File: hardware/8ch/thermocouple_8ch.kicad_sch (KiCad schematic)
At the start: 167 parts, among them J1 24V_INPUT, J2 LCD_16x2_HEADER, J3 RELAY_COM_NO_NC, J4 RS485_A_B_GND_SHIELD, J5 AVR_ISP, J6 MCU_EXPANSION, K1 G5LE-1 DC24, Q1 2N7000, SW1 NEXT, SW2 UP, SW3 DOWN, SW4 SET, SW5 ACK, U1 ATmega32A-PU, U10 ISO7760FDWR, U11 ISO7761FDWR, U12 IA0505S, U13 LP2985-3.3, U14 TSR 1-2450, U15 ADM2587EBRWZ, U2 MAX31856MUD+, U3 MAX31856MUD+, U4 MAX31856MUD+, U5 MAX31856MUD+, U6 MAX31856MUD+, U7 MAX31856MUD+, U8 MAX31856MUD+, U9 MAX31856MUD+

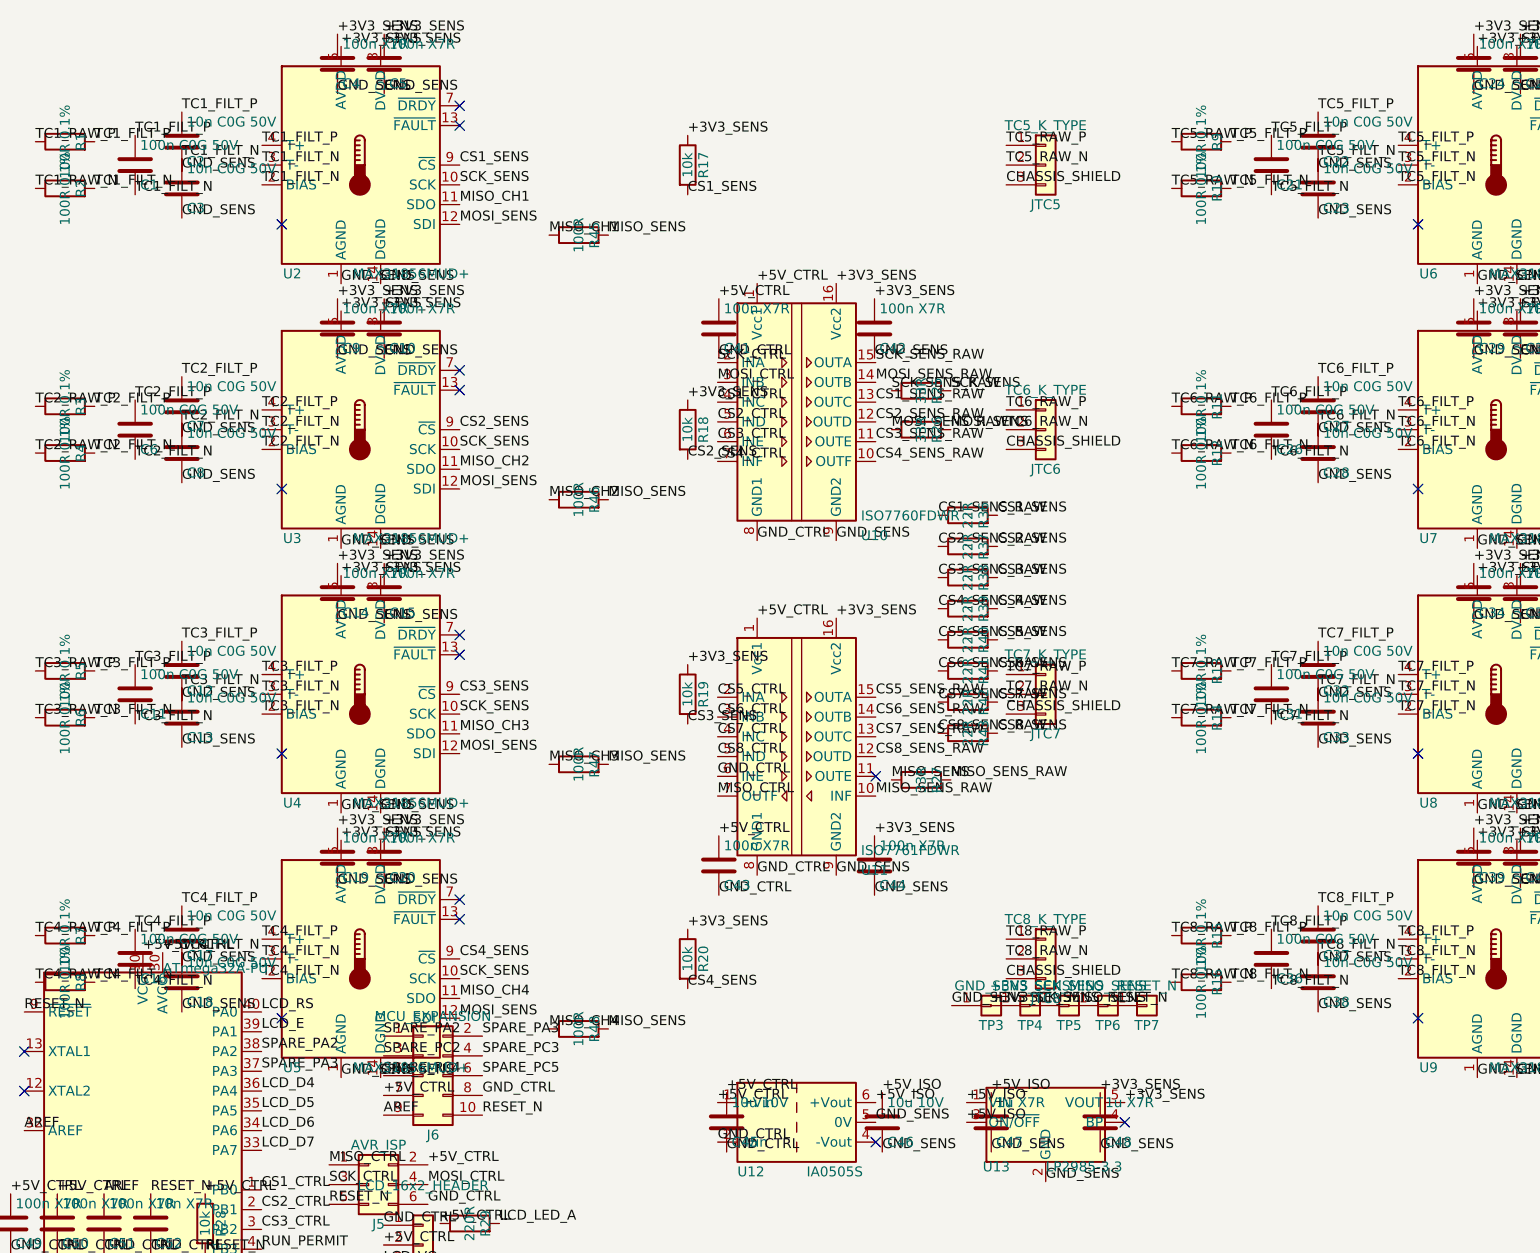
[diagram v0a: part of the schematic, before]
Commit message: tools config
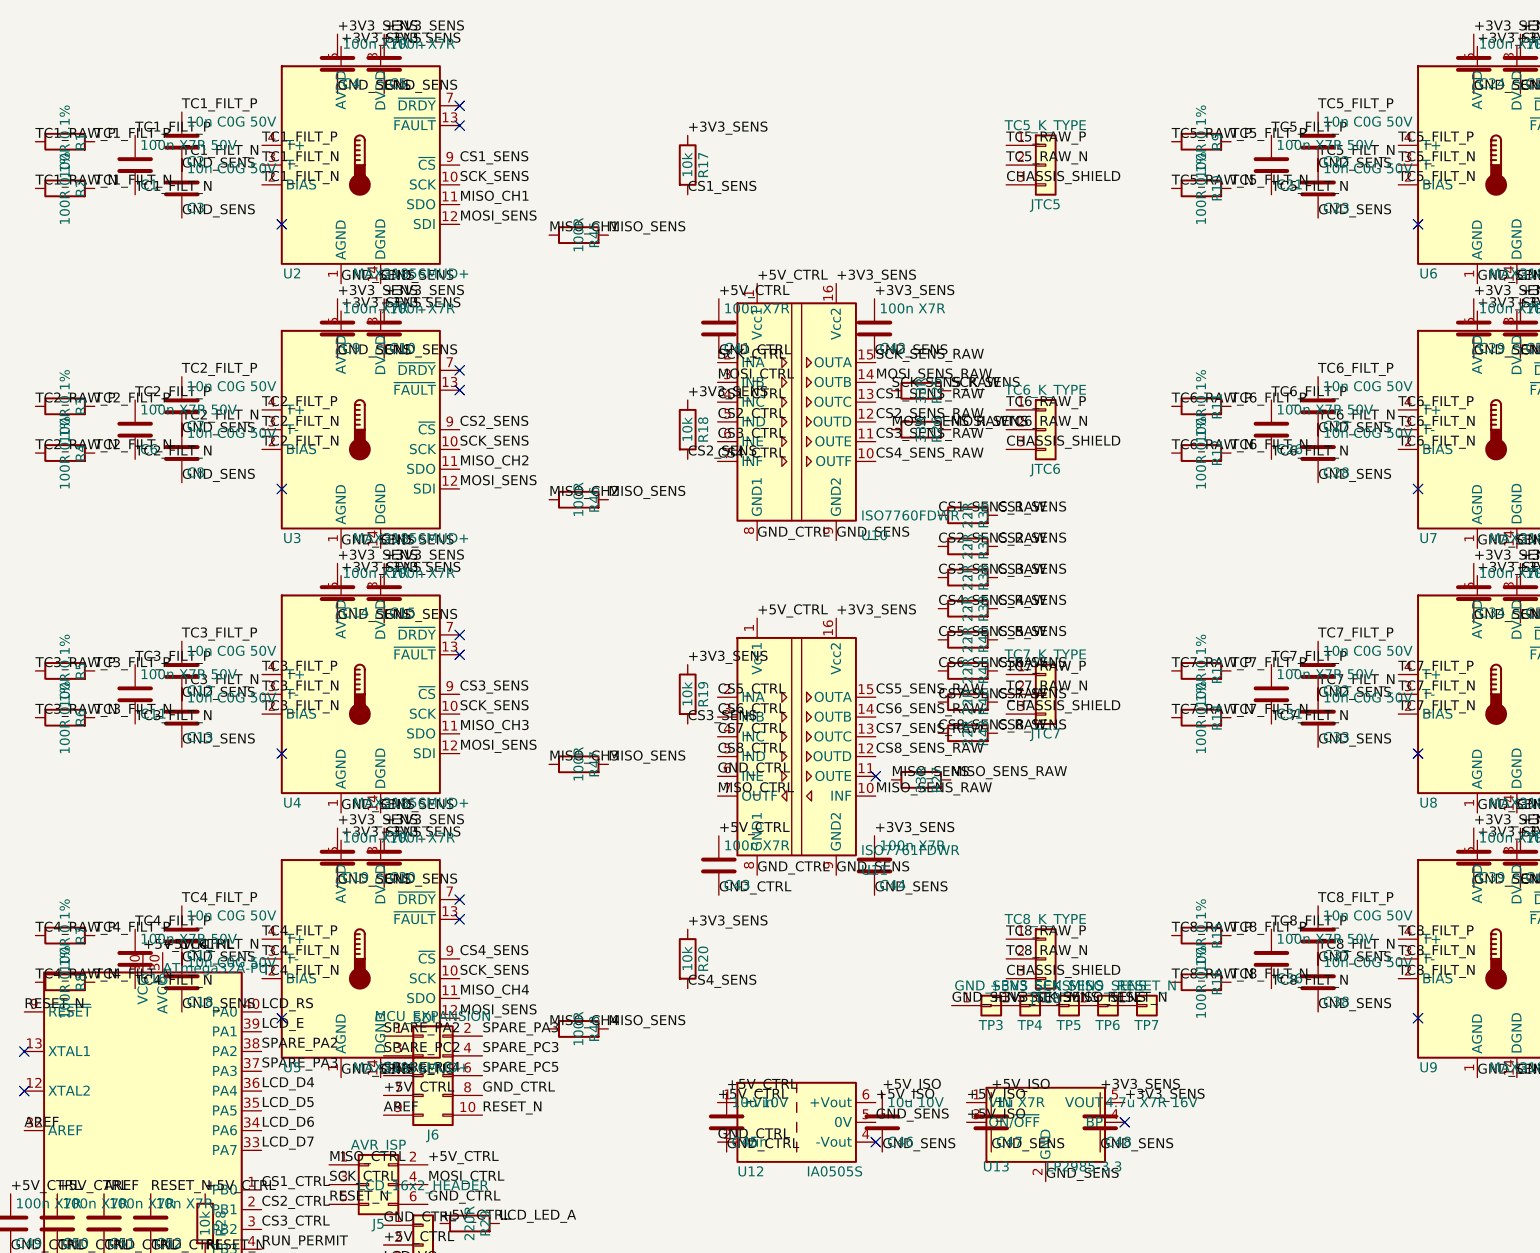
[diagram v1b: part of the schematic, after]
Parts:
- C1, C11, C16, C21, C26, C31, C36, C6: value 100n C0G 50V -> 100n X7R 50V
- C48: value 1u X7R -> 4.7u X7R 16V
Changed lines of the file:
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@@
 			)
 		)
-		(property "Value" "100n C0G 50V"
+		(property "Value" "100n X7R 50V"
 			(at 41.635 19.46 0)
 			(show_name no)
@@
 			)
 		)
-		(property "Value" "1u X7R"
+		(property "Value" "4.7u X7R 16V"
 			(at 165.635 142.46 0)
 			(show_name no)
@@
 			)
 		)
-		(property "Value" "100n C0G 50V"
+		(property "Value" "100n X7R 50V"
 			(at 187.635 121.46 0)
 			(show_name no)
@@
 			)
 		)
-		(property "Value" "100n C0G 50V"
+		(property "Value" "100n X7R 50V"
 			(at 187.635 87.46 0)
 			(show_name no)
@@
 			)
 		)
-		(property "Value" "100n C0G 50V"
+		(property "Value" "100n X7R 50V"
 			(at 187.635 53.46 0)
 			(show_name no)
@@
 			)
 		)
-		(property "Value" "100n C0G 50V"
+		(property "Value" "100n X7R 50V"
 			(at 187.635 19.46 0)
 			(show_name no)
@@
 			)
 		)
-		(property "Value" "100n C0G 50V"
+		(property "Value" "100n X7R 50V"
 			(at 41.635 121.46 0)
 			(show_name no)
@@
 			)
 		)
-		(property "Value" "100n C0G 50V"
+		(property "Value" "100n X7R 50V"
 			(at 41.635 87.46 0)
 			(show_name no)
@@
 			)
 		)
-		(property "Value" "100n C0G 50V"
+		(property "Value" "100n X7R 50V"
 			(at 41.635 53.46 0)
 			(show_name no)

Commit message: 002 schematic
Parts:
- added C60, C61: 22p C0G 50V, Capacitor_SMD:C_0805_2012Metric, symbol Device:C
- added D10, D11, D12, D13, D14, D15, D16, D17, D18, D19, D20, D21, D22, D7, D8, D9: BAV199, Package_TO_SOT_SMD:SOT-23, symbol Device:D_Dual_Series_AKC
- added R53: 22k, Resistor_SMD:R_0805_2012Metric, symbol Device:R
- added R54: 4k7, Resistor_SMD:R_0805_2012Metric, symbol Device:R
- added Y1: 8MHz, Crystal:Crystal_HC49-4H_Vertical, symbol Device:Crystal
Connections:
- net +3V3_SENS: now also D10.2 (K), D11.2 (K), D12.2 (K), D13.2 (K), D14.2 (K), D15.2 (K), D16.2 (K), D17.2 (K), D18.2 (K), D19.2 (K), D20.2 (K), D21.2 (K), D22.2 (K), D7.2 (K), D8.2 (K), D9.2 (K)
- net GND_CTRL: now also C60.2, C61.2, R54.2
- net GND_SENS: now also D10.1 (A), D11.1 (A), D12.1 (A), D13.1 (A), D14.1 (A), D15.1 (A), D16.1 (A), D17.1 (A), D18.1 (A), D19.1 (A), D20.1 (A), D21.1 (A), D22.1 (A), D7.1 (A), D8.1 (A), D9.1 (A)
- net RELAY_LOW: now also R53.1
- net TC1_FILT_N: now also D8.3 (common)
- net TC1_FILT_P: now also D7.3 (common)
- net TC2_FILT_N: now also D10.3 (common)
- net TC2_FILT_P: now also D9.3 (common)
- net TC3_FILT_N: now also D12.3 (common)
- net TC3_FILT_P: now also D11.3 (common)
- net TC4_FILT_N: now also D14.3 (common)
- net TC4_FILT_P: now also D13.3 (common)
- net TC5_FILT_N: now also D16.3 (common)
- net TC5_FILT_P: now also D15.3 (common)
- net TC6_FILT_N: now also D18.3 (common)
- net TC6_FILT_P: now also D17.3 (common)
- net TC7_FILT_N: now also D20.3 (common)
- net TC7_FILT_P: now also D19.3 (common)
- net TC8_FILT_N: now also D22.3 (common)
- net TC8_FILT_P: now also D21.3 (common)
- net XTAL2: now reaches U1.12 (XTAL2)
- net XTAL2: now also C61.1, Y1.2
- net XTAL1: now reaches U1.13 (XTAL1)
- net XTAL1: now also C60.1, Y1.1
- net SPARE_PC2: no longer names the net of J6.3 (Pin_3)
- net SPARE_PC2: no longer U1.24 (PC2)
- new net RUN_PERMIT_SENSE: R53.2, R54.1, U1.24 (PC2)
- no-connect marks 33 -> 32
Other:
- moved on the sheet: C1, C10, C11, C12, C13, C14, C15, C16, C17, C18, C19, C2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

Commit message: push to start cloud
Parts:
- removed U14: TSR 1-2450, Converter_DCDC:Converter_DCDC_TRACO_TSR-1_THT, symbol Converter_DCDC:TSR_1-2450
- added C62: 2.2n 50V X7R, Capacitor_SMD:C_0805_2012Metric, symbol Device:C
- added C63: 4.7u 100V X7R, Capacitor_SMD:C_1210_3225Metric, symbol Device:C
- added C64, C65: 22u 25V X7R, Capacitor_SMD:C_1210_3225Metric, symbol Device:C
- added C67: 3.3n 50V X7R, Capacitor_SMD:C_0805_2012Metric, symbol Device:C
- added C68: 220p C0G 50V, Capacitor_SMD:C_0805_2012Metric, symbol Device:C
- added L1: 33u 2.2A, Inductor_SMD:L_10.4x10.4_H4.8, symbol Device:L
- added R55: 41.2k 1%, Resistor_SMD:R_0805_2012Metric, symbol Device:R
- added R56: 158k 1%, Resistor_SMD:R_0805_2012Metric, symbol Device:R
- added R57: 49.9k 1%, Resistor_SMD:R_0805_2012Metric, symbol Device:R
- added R58: 150k 1%, Resistor_SMD:R_0805_2012Metric, symbol Device:R
- added R59: 33.2k 1%, Resistor_SMD:R_0805_2012Metric, symbol Device:R
- added R60: 10k 1%, Resistor_SMD:R_0805_2012Metric, symbol Device:R
- added U14: LM5164DDAR, Package_SO:SOIC-8-1EP_3.9x4.9mm_P1.27mm_EP2.41x3.3mm_ThermalVias, symbol Regulator_Switching:LM5164DDA
- C1, C10, C11, C14, C15, C16, C19, C20, C21, C24, C25, C26, C29, C30, C31, C34, C35, C36, C39, C4, C40, C41, C42, C43, C44, C49, C5, C50, C51, C56, C58, C6, C9: LCSC (none) -> C49678; MPN (none) -> CC0805KRX7R9BB104
- C12, C13, C17, C18, C2, C22, C23, C27, C28, C3, C32, C33, C37, C38, C7, C8: LCSC (none) -> C97905; MPN (none) -> GRM2195C1H103JA01D
- C45, C46: LCSC (none) -> C15850; MPN (none) -> CL21A106KAYNNNE
- C47: LCSC (none) -> C28323; MPN (none) -> CL21B105KBFNNNE
- C48: LCSC (none) -> C6119943; MPN (none) -> CGA0805X7R475K350MT
- C52: LCSC (none) -> C1710; MPN (none) -> CL21B103KBANNNC
- C53: value 47u 50V -> 22u 100V; footprint Capacitor_THT:CP_Radial_D6.3mm_P2.50mm -> Capacitor_THT:CP_Radial_D8.0mm_P3.50mm; MPN (none) -> EEUFC2A220; Manufacturer (none) -> Panasonic
- C54: value 2.2u 50V X7R -> 4.7u 100V X7R; footprint Capacitor_SMD:C_0805_2012Metric -> Capacitor_SMD:C_1210_3225Metric; LCSC (none) -> C381466; MPN (none) -> FS32X475K101EGG
- C55, C57, C59: LCSC (none) -> C95841; MPN (none) -> CL21B106KOQNNNE
- C60, C61: LCSC (none) -> C1804; MPN (none) -> CL21C220JBANNNC
- D1: value SS34 -> SS310; LCSC (none) -> C15874; MPN (none) -> SS310; Manufacturer (none) -> MDD
- D10, D11, D12, D13, D14, D15, D16, D17, D18, D19, D20, D21, D22, D7, D8, D9: LCSC (none) -> C5184419; MPN (none) -> BAV199; Manufacturer (none) -> Nexperia
- D2: value SMBJ33A -> SMBJ60A; LCSC (none) -> C49066953; MPN (none) -> SMBJ60A; Manufacturer (none) -> MDD
- D3: footprint Diode_THT:D_DO-41_SOD81_P10.16mm_Horizontal -> Diode_SMD:D_SMA; LCSC (none) -> C727081; MPN (none) -> 1N4007; Manufacturer (none) -> MDD
- D4: LCSC (none) -> C52034646; MPN (none) -> 3A4GUD; Manufacturer (none) -> Everlight
- D5, D6: LCSC (none) -> C19077526; MPN (none) -> SMAJ6.0CA; Manufacturer (none) -> Slkor
- F1: LCSC (none) -> C2982267; MPN (none) -> ASMD1206-050-30V; Manufacturer (none) -> Yageo
- J1, J3, JTC1, JTC2, JTC3, JTC4, JTC5, JTC6, JTC7, JTC8: LCSC (none) -> C8270; MPN (none) -> WJ128V-5.0-3P; Manufacturer (none) -> KANGNEX
- J2: LCSC (none) -> C7501270; MPN (none) -> ZX-PZ2.54-1-16PZZ; Manufacturer (none) -> XKB Connection
- J4: LCSC (none) -> C192769; MPN (none) -> WJ128V-5.0-04P-14-00A; Manufacturer (none) -> KANGNEX
- J5: LCSC (none) -> C492420; MPN (none) -> PZ254V-12-6P; Manufacturer (none) -> XKB Connection
- J6: LCSC (none) -> C492422; MPN (none) -> PZ254V-12-10P; Manufacturer (none) -> XKB Connection
- JP1, JP2, JP3: LCSC (none) -> C492401; MPN (none) -> PZ254V-11-02P; Manufacturer (none) -> XKB Connection
- K1: MPN (none) -> G5LE-1 DC24; Manufacturer (none) -> Omron Electronics
- Q1: LCSC (none) -> C9114; MPN (none) -> 2N7000; Manufacturer (none) -> onsemi
- R1, R10, R11, R12, R13, R14, R15, R16, R2, R3, R4, R5, R6, R7, R8, R9: LCSC (none) -> C110773; MPN (none) -> RT0805BRD07100RL
- R17, R18, R19, R20, R21, R22, R23, R24, R28: LCSC (none) -> C17414; MPN (none) -> 0805W8F1002T5E
- R25, R26, R27: LCSC (none) -> C17634; MPN (none) -> 0805W8F330JT5E
- R29: LCSC (none) -> C17557; MPN (none) -> 0805W8F2200T5E
- R30, R45, R46, R47, R48, R49, R50, R51, R52: LCSC (none) -> C17408; MPN (none) -> 0805W8F1000T5E
- R31: LCSC (none) -> C149504; MPN (none) -> 0805W8F1003T5E
- R32: LCSC (none) -> C276229; MPN (none) -> RK73H2ATTD4701F
- R33: LCSC (none) -> C17477; MPN (none) -> 0805W8F0000T5E
- R34: LCSC (none) -> C17437; MPN (none) -> 0805W8F1200T5E
- R35, R44: LCSC (none) -> C17798; MPN (none) -> 0805W8F6800T5E
- R36, R37, R38, R39, R40, R41, R42, R43: LCSC (none) -> C17561; MPN (none) -> 0805W8F220JT5E
- R53: LCSC (none) -> C17560; MPN (none) -> 0805W8F2202T5E
- R54: LCSC (none) -> C17673; MPN (none) -> 0805W8F4701T5E
- RV1: MPN (none) -> 3296W-1-103LF; Manufacturer (none) -> Bourns
- SW1, SW2, SW3, SW4, SW5: LCSC (none) -> C393938; MPN (none) -> TS665CJ; Manufacturer (none) -> XKB Connection
- U1: MPN (none) -> ATMEGA32A-PU; Manufacturer (none) -> Microchip Technology
- U10: MPN (none) -> ISO7760FDWR; Manufacturer (none) -> Texas Instruments
- U11: MPN (none) -> ISO7761FDWR; Manufacturer (none) -> Texas Instruments
- U12: MPN (none) -> IA0505S; Manufacturer (none) -> XP Power
- U13: MPN (none) -> LP2985IM5X-3.3/NOPB; Manufacturer (none) -> Texas Instruments
- U15: MPN (none) -> ADM2587EBRWZ; Manufacturer (none) -> Analog Devices
- U2, U3, U4, U5, U6, U7, U8, U9: MPN (none) -> MAX31856MUD+; Manufacturer (none) -> Analog Devices
- Y1: value 8MHz -> 8MHz 20pF; footprint Crystal:Crystal_HC49-4H_Vertical -> Crystal:Crystal_SMD_HC49-SD; LCSC (none) -> C12674; MPN (none) -> X49SM8MSD2SC; Manufacturer (none) -> Yangxing Tech
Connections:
- net +24V_PROT: now also C63.1, R59.1, U14.2 (VIN)
- net +5V_CTRL: now also C64.1, C65.1, C67.2, L1.2, R56.1
- net GND_CTRL: now also C63.2, C64.2, C65.2, R55.2, R57.2, R60.2, U14.1 (GND), U14.9 (EP)
- new net BST_5V: C62.1, U14.7 (BST)
- new net FB_5V: C68.2, R56.2, R57.1, U14.5 (FB)
- new net RIPPLE_INJ: C67.1, C68.1, R58.2
- new net RON_SET: R55.1, U14.4 (RON)
- new net SW_5V: C62.2, L1.1, R58.1, U14.8 (SW)
- new net VIN_UVLO: R59.2, R60.1, U14.3 (EN/UVLO)
- no-connect marks 32 -> 33
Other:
- moved on the sheet: JTC1, JTC2, JTC3, JTC4, R1, R10, R12, R14, R15, R16, R2, R4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

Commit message: Redraw the schematic with wires (I-002), fix the K1 relay coil pins (I-058) and the U12 symbol link (I-057).
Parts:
- U12: symbol Converter_DCDC:IA0305S -> Converter_DCDC_Isolated:IA0505S
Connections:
- net RELAY_COM: now also K1.1; no longer K1.4
- net RELAY_LOW: now also K1.5; no longer K1.1
- net RELAY_NC: now also K1.4; no longer K1.5
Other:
- moved on the sheet: C1, C10, C11, C12, C13, C14, C15, C16, C17, C18, C19, C2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
